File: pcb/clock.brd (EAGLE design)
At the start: 113.3 x 50.6 mm, 89 parts, among them Q1 BC849SMD, Q10 BC847BSMD, Q11 BC849SMD, Q12 BC849SMD, Q13 BC849SMD, Q14 BC857BSMD, Q15 BC847BSMD, Q16 BC857BSMD, Q17 BC847BSMD, Q18 BC857BSMD, Q19 BC847BSMD, Q2 BC849SMD, Q20 BC857BSMD, Q21 BC847BSMD, Q22 BC857BSMD, Q23 BC847BSMD, Q24 BC857BSMD, Q3 BC849SMD, Q4 BC849SMD, Q5 BC849SMD, Q6 BC849SMD, Q7 BC849SMD, Q8 BC849SMD, Q9 BC849SMD, U2 ATXMEGA16D4-AU, X1 MINI-USB-32005-301

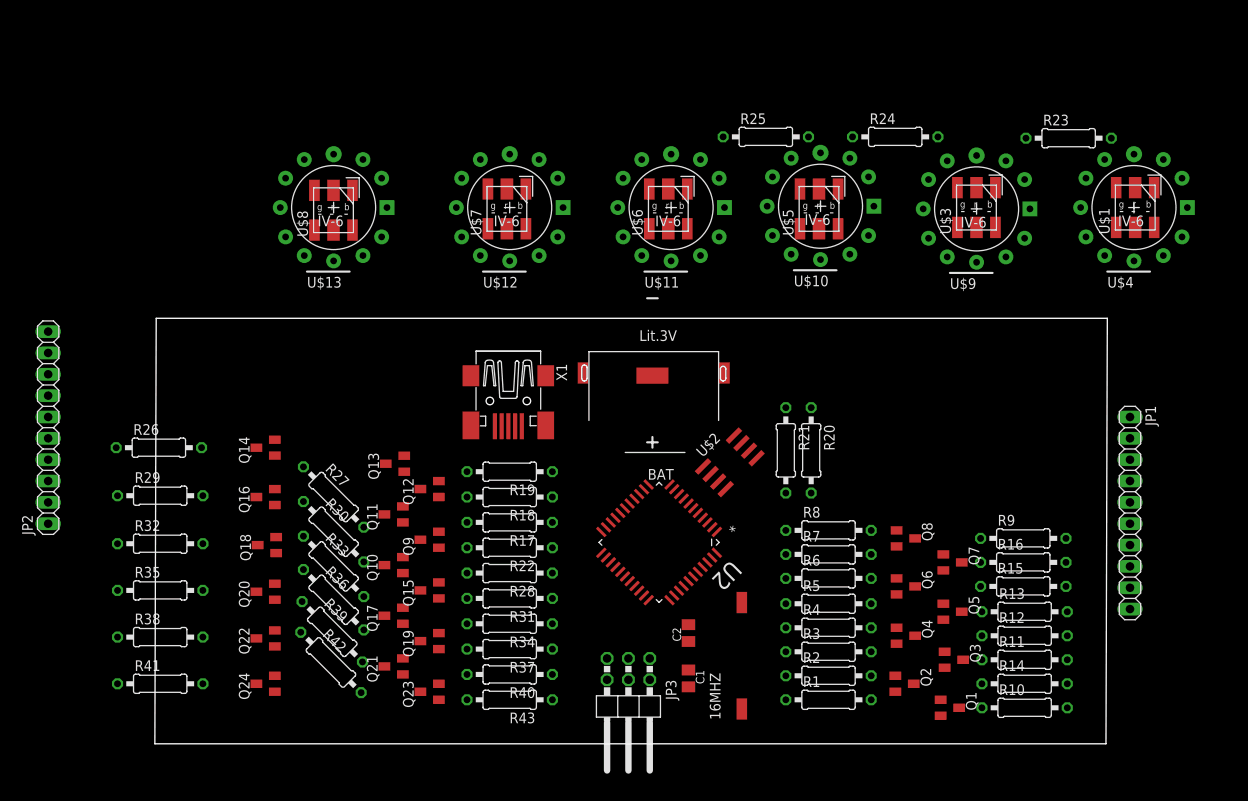
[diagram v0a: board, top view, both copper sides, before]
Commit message: funkcni prototyp
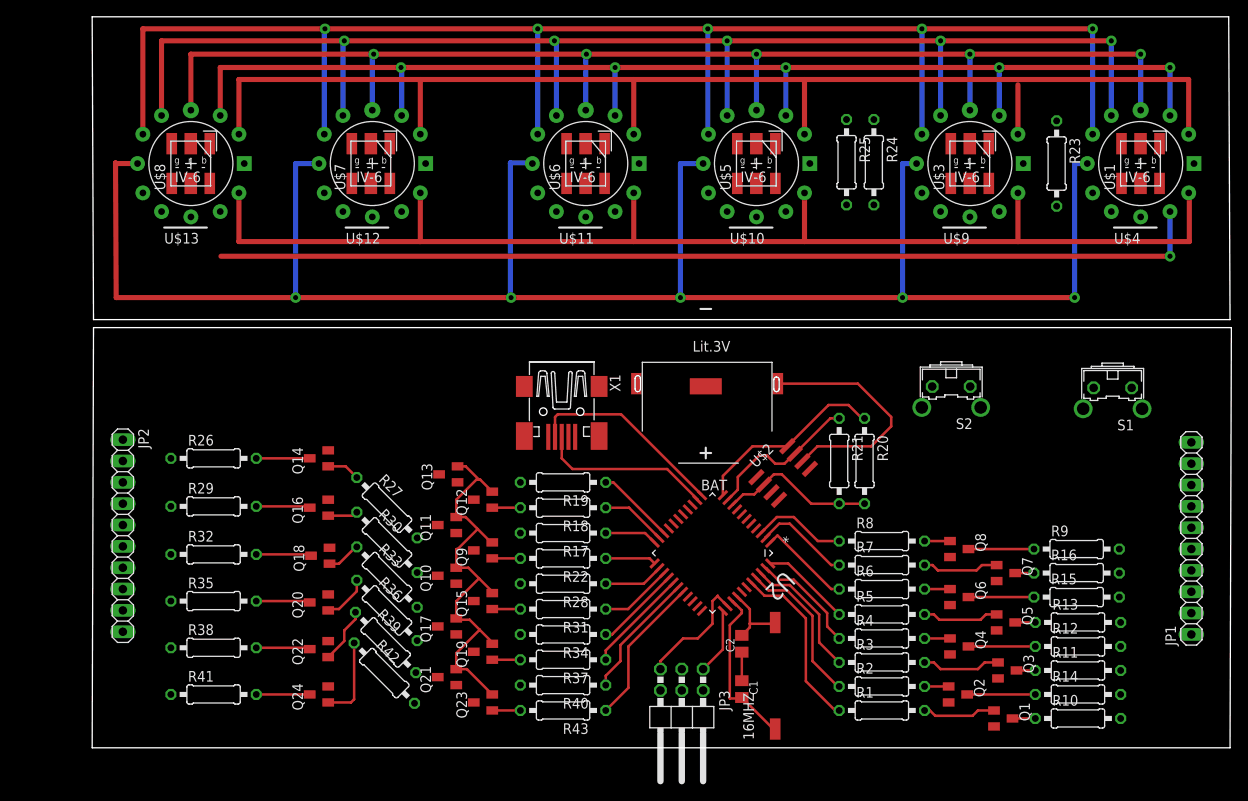
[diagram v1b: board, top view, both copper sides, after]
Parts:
- added S1, S2: (no value), switch-omron:B3F-31XX
- moved U$8 17.9 mm to (-95.1, 40.8)
- moved U$13 17.8 mm to (-92.7, 43.3)
- moved U$12 17.2 mm to (-71.1, 43.3)
- moved U$7 17.1 mm to (-73.7, 40.8)
- moved JP2 15.6 mm to (-100.8, -0.95), turned to 270 degrees
- moved U$11 11.4 mm to (-45.7, 43.3)
- moved U$6 11.2 mm to (-48.1, 40.8)
- moved R25 10.1 mm to (-14.7, 43.5), turned to 270 degrees
- moved U$5 9.21 mm to (-27.8, 40.8)
- moved U$10 9.16 mm to (-25.4, 43.3)
- moved JP1 7.90 mm to (26.4, -1.27), turned to 90 degrees
- moved R26 6.63 mm to (-90.0, 8.26)
- moved R42 6.48 mm to (-69.7, -17.3)
- moved C1 6.48 mm to (-27.1, -19.2)
- moved C2 6.48 mm to (-27.1, -13.8)
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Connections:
- new net BL: U$10.BL, U$11.BL, U$12.BL, U$13.BL, U$4.BL, U$9.BL
- new net BOT: U$10.BOT, U$11.BOT, U$12.BOT, U$13.BOT, U$4.BOT, U$9.BOT
- new net BR: U$10.BR, U$11.BR, U$12.BR, U$13.BR, U$4.BR, U$9.BR
- new net DOT: U$10.DOT, U$11.DOT, U$12.DOT, U$13.DOT, U$4.DOT, U$9.DOT
- new net FIL_P: U$10.FIL_P, U$11.FIL_P, U$12.FIL_P, U$13.FIL_P, U$4.FIL_P, U$9.FIL_P
- new net MID: U$10.MID, U$11.MID, U$12.MID, U$13.MID, U$4.MID, U$9.MID
- new net N$54: U$4.FIL_M
- new net N$63: U$9.FIL_M
- new net N$68: U$11.GRID_P
- new net N$69: U$11.FIL_M
- new net N$70: U$10.GRID_P
- new net N$71: U$10.FIL_M
- new net N$72: U$4.GRID_P
- new net N$73: U$9.GRID_P
- new net N$74: U$12.GRID_P
- new net N$76: U$12.FIL_M
- new net N$77: U$13.GRID_P
- new net N$79: U$13.FIL_M
- new net TL: U$10.TL, U$11.TL, U$12.TL, U$13.TL, U$4.TL, U$9.TL
- new net TOP: U$10.TOP, U$11.TOP, U$12.TOP, U$13.TOP, U$4.TOP, U$9.TOP
- new net TR: U$10.TR, U$11.TR, U$12.TR, U$13.TR, U$4.TR, U$9.TR
- net G: now also U$5.KB
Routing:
- net BOT: track 0.00 -> 224.0 mm, vias 0 -> 5
- net BL: track 0.00 -> 188.4 mm, vias 0 -> 5
- net TL: track 0.00 -> 166.5 mm, vias 0 -> 5
- net MID: track 0.00 -> 153.1 mm, vias 0 -> 5
- net TR: track 0.00 -> 151.4 mm
- net DOT: track 0.00 -> 148.0 mm
- net TOP: track 0.00 -> 147.4 mm, vias 0 -> 5
- net BR: track 0.00 -> 118.3 mm, vias 0 -> 1
- net GND: track 0.00 -> 54.4 mm
- net N$28: track 0.00 -> 28.5 mm
- net RX: track 0.00 -> 24.0 mm
- net N$25: track 0.00 -> 23.3 mm
- net PA0: track 0.00 -> 21.1 mm
- net TX: track 0.00 -> 20.8 mm
- net N$5: track 0.00 -> 19.6 mm
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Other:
- board size 113.3 x 50.6 mm -> 135.6 x 87 mm
